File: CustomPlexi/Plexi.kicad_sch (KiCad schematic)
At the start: 24 parts, among them SW1 Diode Select, SW2 Clipping Type, SW5 Plexi Channel Select, U1 TL074

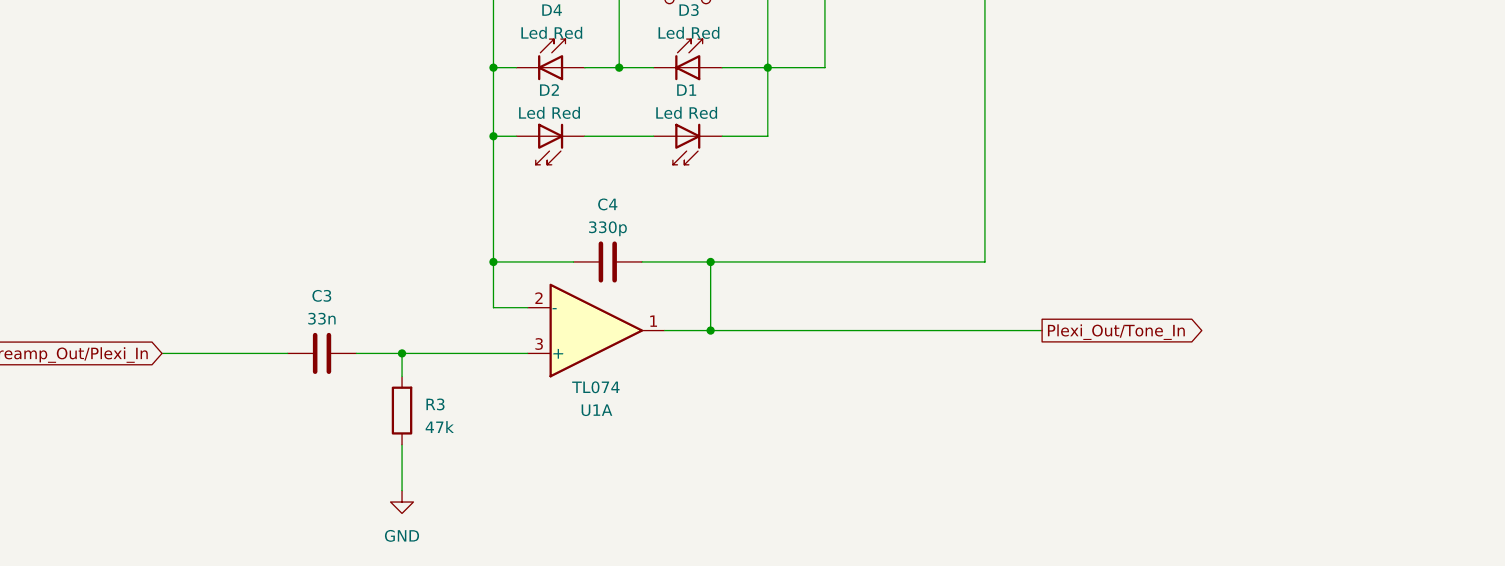
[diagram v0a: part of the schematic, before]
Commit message: commit
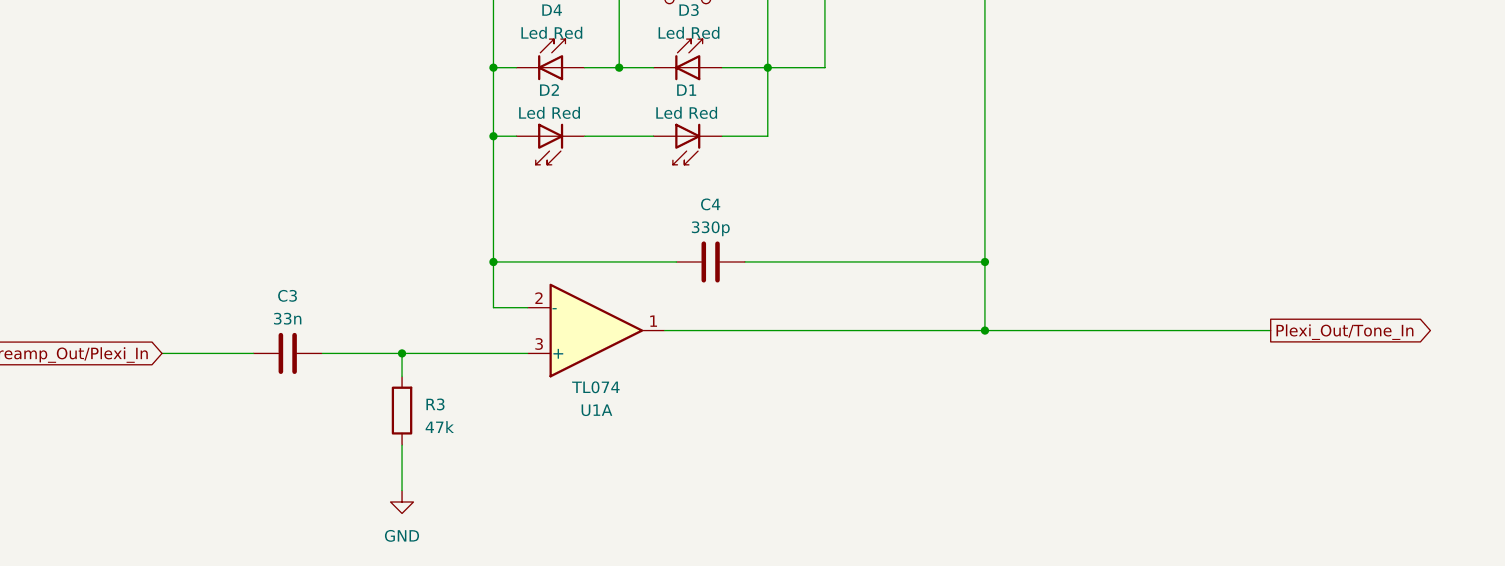
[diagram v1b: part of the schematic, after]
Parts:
- C3, C4: footprint Capacitor_SMD_AKL:C_0603_1608Metric -> Capacitor_SMD:C_0402_1005Metric_Pad0.74x0.62mm_HandSolder
- R3, R4, R5: footprint Resistor_SMD_AKL:R_0603_1608Metric -> Resistor_SMD:R_0402_1005Metric_Pad0.72x0.64mm_HandSolder
- RV1, RV2: footprint (none) -> PCM_Potentiometer_THT_US_AKL_Double:Potentiometer_Vishay_148-149_Single_Vertical
- SW1, SW2: footprint (none) -> CustomLib:SW_SP3T_PinHeader2.54mm
- SW5: footprint (none) -> CustomLib:SW_SPST_x4_PinHeader2.54mm
- U1: footprint (none) -> Package_SO:SOIC-14W_7.5x9mm_P1.27mm
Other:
- moved on the sheet: C3, C4
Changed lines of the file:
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@@
   (junction (at 110.49 140.97) (diameter 0) (color 0 0 0 0)
   )
-  (junction (at 134.62 140.97) (diameter 0) (color 0 0 0 0)
-  )
   (junction (at 110.49 41.91) (diameter 0) (color 0 0 0 0)
   )
-  (junction (at 134.62 148.59) (diameter 0) (color 0 0 0 0)
+  (junction (at 165.1 140.97) (diameter 0) (color 0 0 0 0)
+  )
+  (junction (at 165.1 148.59) (diameter 0) (color 0 0 0 0)
   )
   (junction (at 110.49 95.25) (diameter 0) (color 0 0 0 0)
@@
     (stroke (width 0) (type default))
   )
-  (wire (pts (xy 73.66 151.13) (xy 87.63 151.13))
+  (wire (pts (xy 73.66 151.13) (xy 83.82 151.13))
     (stroke (width 0) (type default))
   )
@@
     (stroke (width 0) (type default))
   )
-  (wire (pts (xy 110.49 140.97) (xy 119.38 140.97))
+  (wire (pts (xy 110.49 140.97) (xy 130.81 140.97))
     (stroke (width 0) (type default))
   )
@@
     (stroke (width 0) (type default))
   )
-  (wire (pts (xy 134.62 140.97) (xy 134.62 148.59))
-    (stroke (width 0) (type default))
-  )
-  (wire (pts (xy 134.62 140.97) (xy 165.1 140.97))
-    (stroke (width 0) (type default))
-  )
   (wire (pts (xy 110.49 146.05) (xy 110.49 140.97))
     (stroke (width 0) (type default))
@@
     (stroke (width 0) (type default))
   )
-  (wire (pts (xy 95.25 151.13) (xy 100.33 151.13))
+  (wire (pts (xy 91.44 151.13) (xy 100.33 151.13))
     (stroke (width 0) (type default))
   )
@@
     (stroke (width 0) (type default))
   )
+  (wire (pts (xy 165.1 148.59) (xy 196.85 148.59))
+    (stroke (width 0) (type default))
+  )
   (wire (pts (xy 110.49 102.87) (xy 113.03 102.87))
     (stroke (width 0) (type default))
@@
     (stroke (width 0) (type default))
   )
-  (wire (pts (xy 134.62 148.59) (xy 129.54 148.59))
-    (stroke (width 0) (type default))
-  )
   (wire (pts (xy 135.89 69.85) (xy 140.97 69.85))
     (stroke (width 0) (type default))
@@
     (stroke (width 0) (type default))
   )
-  (wire (pts (xy 134.62 148.59) (xy 171.45 148.59))
+  (wire (pts (xy 129.54 148.59) (xy 165.1 148.59))
     (stroke (width 0) (type default))
   )
@@
     (stroke (width 0) (type default))
   )
-  (wire (pts (xy 127 140.97) (xy 134.62 140.97))
+  (wire (pts (xy 138.43 140.97) (xy 165.1 140.97))
     (stroke (width 0) (type default))
   )
@@
   )
   (wire (pts (xy 97.79 60.96) (xy 97.79 63.5))
+    (stroke (width 0) (type default))
+  )
+  (wire (pts (xy 165.1 140.97) (xy 165.1 148.59))
     (stroke (width 0) (type default))
   )
@@
     )
   )
-  (global_label "Plexi_Out{slash}Tone_In" (shape output) (at 171.45 148.59 0) (fields_autoplaced)
+  (global_label "Plexi_Out{slash}Tone_In" (shape output) (at 196.85 148.59 0) (fields_autoplaced)
     (effects (font (size 1.27 1.27)) (justify left))
-    (property "Intersheetrefs" "${INTERSHEET_REFS}" (at 191.5914 148.59 0)
+    (property "Intersheetrefs" "${INTERSHEET_REFS}" (at 216.9914 148.59 0)
       (effects (font (size 1.27 1.27)) (justify left) hide)
     )
@@
       (effects (font (size 1.27 1.27)) (justify right))
     )
-    (property "Footprint" "Resistor_SMD_AKL:R_0603_1608Metric" (at 97.79 33.02 0)
+    (property "Footprint" "Resistor_SMD:R_0402_1005Metric_Pad0.72x0.64mm_HandSolder" (at 97.79 33.02 0)
       (effects (font (size 1.27 1.27)) hide)
     )
@@
       (effects (font (size 1.27 1.27)))
     )
-    (property "Footprint" "" (at 120.65 151.13 0)
+    (property "Footprint" "Package_SO:SOIC-14W_7.5x9mm_P1.27mm" (at 120.65 151.13 0)
       (effects (font (size 1.27 1.27)) hide)
     )
@@
       (effects (font (size 1.27 1.27)))
     )
-    (property "Footprint" "" (at 123.19 36.83 0)
+    (property "Footprint" "PCM_Potentiometer_THT_US_AKL_Double:Potentiometer_Vishay_148-149_Single_Vertical" (at 123.19 36.83 0)
       (effects (font (size 1.27 1.27)) hide)
     )
@@
       (effects (font (size 1.27 1.27)))
     )
-    (property "Footprint" "Resistor_SMD_AKL:R_0603_1608Metric" (at 165.1 55.88 0)
+    (property "Footprint" "Resistor_SMD:R_0402_1005Metric_Pad0.72x0.64mm_HandSolder" (at 165.1 55.88 0)
       (effects (font (size 1.27 1.27)) hide)
     )
@@
       (effects (font (size 1.27 1.27)))
     )
-    (property "Footprint" "" (at 128.27 110.49 0)
+    (property "Footprint" "CustomLib:SW_SP3T_PinHeader2.54mm" (at 128.27 110.49 0)
       (effects (font (size 1.27 1.27)) hide)
     )
@@
     )
   )
-  (symbol (lib_id "PCM_Capacitor_AKL:C_0603") (at 123.19 140.97 90) (unit 1)
-    (in_bom yes) (on_board yes) (dnp no)
-    (property "Reference" "C4" (at 123.19 134.62 90)
-      (effects (font (size 1.27 1.27)))
-    )
-    (property "Value" "330p" (at 123.19 137.16 90)
-      (effects (font (size 1.27 1.27)))
-    )
-    (property "Footprint" "Capacitor_SMD_AKL:C_0603_1608Metric" (at 127 140.0048 0)
-      (effects (font (size 1.27 1.27)) hide)
-    )
-    (property "Datasheet" "~" (at 123.19 140.97 0)
+  (symbol (lib_id "PCM_Capacitor_AKL:C_0603") (at 134.62 140.97 90) (unit 1)
+    (in_bom yes) (on_board yes) (dnp no)
+    (property "Reference" "C4" (at 134.62 134.62 90)
+      (effects (font (size 1.27 1.27)))
+    )
+    (property "Value" "330p" (at 134.62 137.16 90)
+      (effects (font (size 1.27 1.27)))
+    )
+    (property "Footprint" "Capacitor_SMD:C_0402_1005Metric_Pad0.74x0.62mm_HandSolder" (at 138.43 140.0048 0)
+      (effects (font (size 1.27 1.27)) hide)
+    )
+    (property "Datasheet" "~" (at 134.62 140.97 0)
       (effects (font (size 1.27 1.27)) hide)
     )
@@
       (effects (font (size 1.27 1.27)))
     )
-    (property "Footprint" "" (at 152.4 38.1 0)
+    (property "Footprint" "CustomLib:SW_SPST_x4_PinHeader2.54mm" (at 152.4 38.1 0)
       (effects (font (size 1.27 1.27)) hide)
     )
@@
       (effects (font (size 1.27 1.27)))
     )
-    (property "Footprint" "" (at 128.27 86.36 0)
+    (property "Footprint" "CustomLib:SW_SP3T_PinHeader2.54mm" (at 128.27 86.36 0)
       (effects (font (size 1.27 1.27)) hide)
     )
@@
       (effects (font (size 1.27 1.27)) (justify right))
     )
-    (property "Footprint" "Resistor_SMD_AKL:R_0603_1608Metric" (at 100.33 146.05 0)
+    (property "Footprint" "Resistor_SMD:R_0402_1005Metric_Pad0.72x0.64mm_HandSolder" (at 100.33 146.05 0)
       (effects (font (size 1.27 1.27)) hide)
     )
@@
       (effects (font (size 1.27 1.27)))
     )
-    (property "Footprint" "" (at 172.085 90.805 0)
+    (property "Footprint" "CustomLib:SW_SP3T_PinHeader2.54mm" (at 172.085 90.805 0)
       (effects (font (size 1.27 1.27)) hide)
     )
@@
       (effects (font (size 1.27 1.27)))
     )
-    (property "Footprint" "" (at 129.54 60.96 0)
+    (property "Footprint" "CustomLib:SW_SP3T_PinHeader2.54mm" (at 129.54 60.96 0)
       (effects (font (size 1.27 1.27)) hide)
     )
@@
     )
   )
-  (symbol (lib_id "PCM_Capacitor_AKL:C_0603") (at 91.44 151.13 90) (unit 1)
-    (in_bom yes) (on_board yes) (dnp no) (fields_autoplaced)
-    (property "Reference" "C3" (at 91.44 144.78 90)
-      (effects (font (size 1.27 1.27)))
-    )
-    (property "Value" "33n" (at 91.44 147.32 90)
-      (effects (font (size 1.27 1.27)))
-    )
-    (property "Footprint" "Capacitor_SMD_AKL:C_0603_1608Metric" (at 95.25 150.1648 0)
-      (effects (font (size 1.27 1.27)) hide)
-    )
-    (property "Datasheet" "~" (at 91.44 151.13 0)
+  (symbol (lib_id "PCM_Capacitor_AKL:C_0603") (at 87.63 151.13 90) (unit 1)
+    (in_bom yes) (on_board yes) (dnp no) (fields_autoplaced)
+    (property "Reference" "C3" (at 87.63 144.78 90)
+      (effects (font (size 1.27 1.27)))
+    )
+    (property "Value" "33n" (at 87.63 147.32 90)
+      (effects (font (size 1.27 1.27)))
+    )
+    (property "Footprint" "Capacitor_SMD:C_0402_1005Metric_Pad0.74x0.62mm_HandSolder" (at 91.44 150.1648 0)
+      (effects (font (size 1.27 1.27)) hide)
+    )
+    (property "Datasheet" "~" (at 87.63 151.13 0)
       (effects (font (size 1.27 1.27)) hide)
     )
@@
       (effects (font (size 1.27 1.27)))
     )
-    (property "Footprint" "" (at 123.19 49.53 0)
-      (effects (font (size 1.27 1.27)) hide)
-    )
+    (property "Footprint" "PCM_Potentiometer_THT_US_AKL_Double:Potentiometer_Vishay_148-149_Single_Vertical" (at 123.19 49.53 0)
+      (effects (font (size 1.27 1.27)) hide)
+    )
